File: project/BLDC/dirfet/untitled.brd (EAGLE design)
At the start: 50 x 47 mm, 64 parts, among them IC1 OPA340N, IC2 INA168, IC3 stm32, IC4 LM258DG, Q1 DFET, Q2 DFET, Q3 DFET, Q4 DFET, Q5 DFET, Q6 DFET

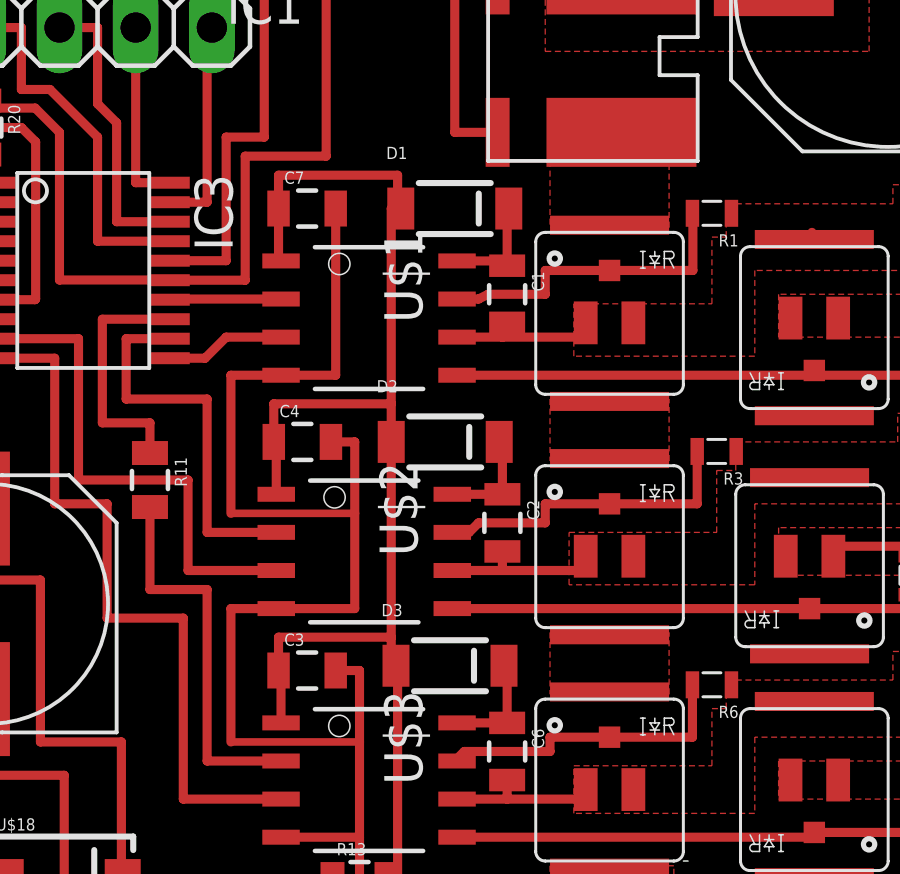
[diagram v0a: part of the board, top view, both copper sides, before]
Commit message: fix lbr(add2)
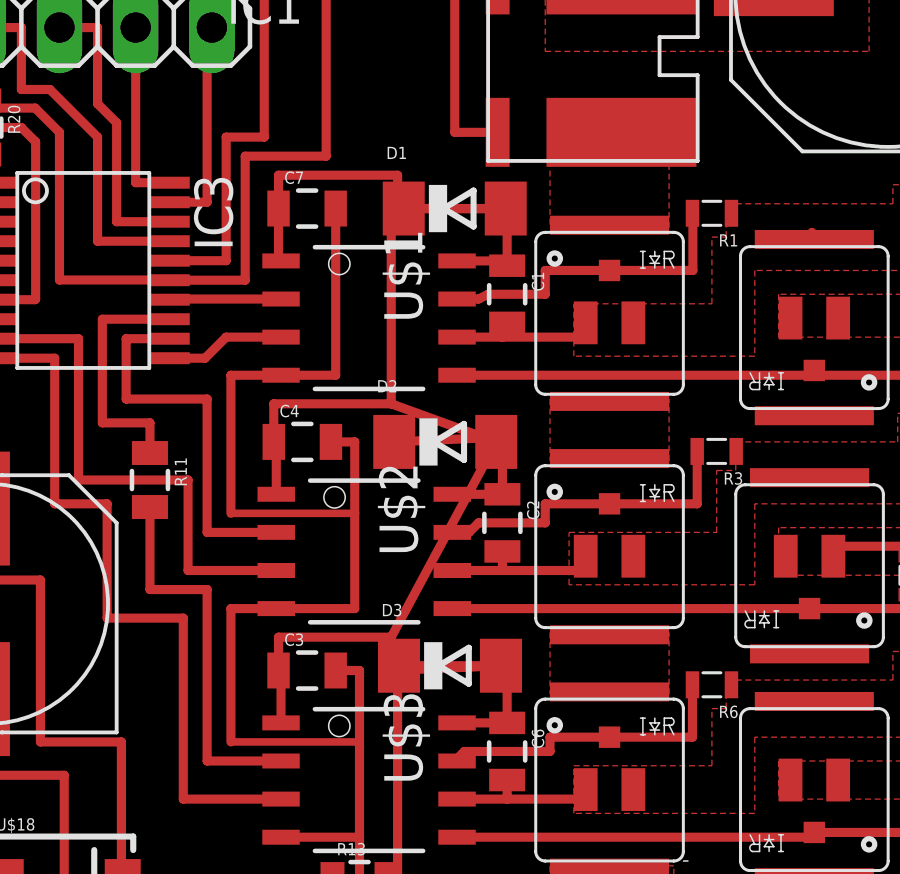
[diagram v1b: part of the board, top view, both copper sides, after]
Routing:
- net 12V: track 45.3 -> 62.5 mm
- net N$7: track 3.68 -> 7.18 mm
- net N$2: track 3.77 -> 7.18 mm
- net N$5: track 3.67 -> 7.06 mm
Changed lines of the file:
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@@
 <contactref element="U$1" pad="8"/>
 <contactref element="C1" pad="1"/>
-<wire x1="30.375" y1="33.9725" x2="30.32125" y2="33.9725" width="0.3048" layer="1"/>
+<wire x1="26.875" y1="33.9725" x2="30.32125" y2="33.9725" width="0.3048" layer="1"/>
 <wire x1="30.32125" y1="33.9725" x2="30.32125" y2="32.0675" width="0.3048" layer="1"/>
 <wire x1="28.6512" y1="32.22625" x2="30.00375" y2="32.22625" width="0.3048" layer="1"/>
@@
 <contactref element="U$3" pad="1"/>
 <contactref element="C7" pad="1"/>
-<wire x1="26.61625" y1="18.7325" x2="26.4575" y2="18.57375" width="0.3048" layer="1"/>
+<wire x1="30.11625" y1="18.7325" x2="26.4575" y2="18.57375" width="0.3048" layer="1"/>
 <wire x1="26.4575" y1="18.57375" x2="26.4575" y2="19.685" width="0.3048" layer="1"/>
-<wire x1="26.4575" y1="19.685" x2="26.4575" y2="26.19375" width="0.3048" layer="1"/>
-<wire x1="26.775" y1="33.9725" x2="26.4575" y2="33.9725" width="0.3048" layer="1"/>
+<wire x1="26.4575" y1="19.685" x2="29.9575" y2="26.19375" width="0.3048" layer="1"/>
+<wire x1="30.275" y1="33.9725" x2="26.4575" y2="33.9725" width="0.3048" layer="1"/>
 <wire x1="26.4575" y1="33.9725" x2="26.4575" y2="27.46375" width="0.3048" layer="1"/>
-<wire x1="26.4575" y1="27.46375" x2="26.4575" y2="26.19375" width="0.3048" layer="1"/>
+<wire x1="26.4575" y1="27.46375" x2="29.9575" y2="26.19375" width="0.3048" layer="1"/>
 <wire x1="22.7838" y1="32.22625" x2="22.70125" y2="32.22625" width="0.3048" layer="1"/>
 <wire x1="22.70125" y1="32.22625" x2="22.70125" y2="33.9725" width="0.3048" layer="1"/>
-<wire x1="26.775" y1="33.9725" x2="26.67" y2="33.9725" width="0.3048" layer="1"/>
+<wire x1="30.275" y1="33.9725" x2="26.67" y2="33.9725" width="0.3048" layer="1"/>
 <wire x1="26.67" y1="33.9725" x2="26.67" y2="35.08375" width="0.3048" layer="1"/>
 <wire x1="26.67" y1="35.08375" x2="22.70125" y2="35.08375" width="0.3048" layer="1"/>
@@
 <wire x1="26.3" y1="11.58875" x2="26.67" y2="11.58875" width="0.3048" layer="1"/>
 <wire x1="26.67" y1="11.58875" x2="26.67" y2="18.7325" width="0.3048" layer="1"/>
-<wire x1="26.67" y1="18.7325" x2="26.61625" y2="18.7325" width="0.254" layer="1"/>
+<wire x1="26.67" y1="18.7325" x2="30.11625" y2="18.7325" width="0.254" layer="1"/>
 </signal>
 <signal name="N$1">
@@
 <contactref element="U$2" pad="8"/>
 <contactref element="C2" pad="1"/>
-<wire x1="30.0575" y1="26.19375" x2="30.1625" y2="26.3525" width="0.3048" layer="1"/>
+<wire x1="26.5575" y1="26.19375" x2="30.1625" y2="26.3525" width="0.3048" layer="1"/>
 <wire x1="30.1625" y1="26.3525" x2="30.1625" y2="24.4475" width="0.3048" layer="1"/>
 <wire x1="28.49245" y1="24.4475" x2="30.1625" y2="24.4475" width="0.3048" layer="1"/>
@@
 <contactref element="C6" pad="1"/>
 <wire x1="30.32125" y1="16.8275" x2="28.6512" y2="16.8275" width="0.3048" layer="1"/>
-<wire x1="30.21625" y1="18.7325" x2="30.32125" y2="18.7325" width="0.3048" layer="1"/>
+<wire x1="26.71625" y1="18.7325" x2="30.32125" y2="18.7325" width="0.3048" layer="1"/>
 <wire x1="30.32125" y1="18.7325" x2="30.32125" y2="16.8275" width="0.3048" layer="1"/>
 </signal>
